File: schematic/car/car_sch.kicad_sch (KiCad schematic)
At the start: 12 parts, among them J1 Led, J10 Motor-PWR-IN, J2 Servo, J3 NRF-Power, J4 Accel, J5 Micro-Power-IN, J6 MOTOR-CTRL, J7 MOTOR-PWR-OUT, J8 Horn, J9 Powers, U1 ARDUINO_PRO_MINI, U2 NRF24L01_Breakout

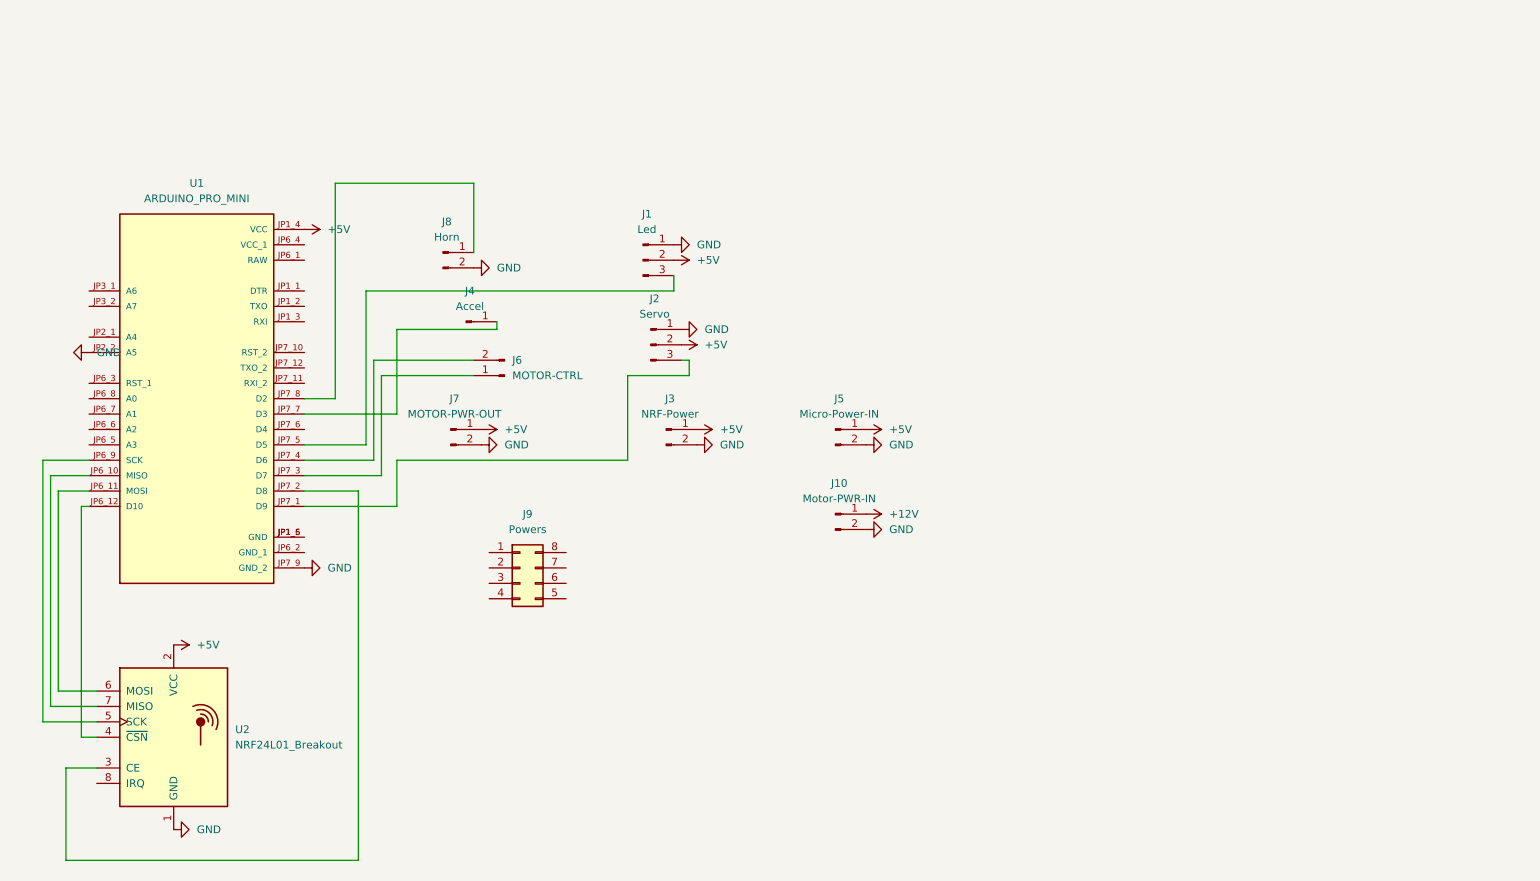
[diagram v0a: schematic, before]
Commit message: drv8833
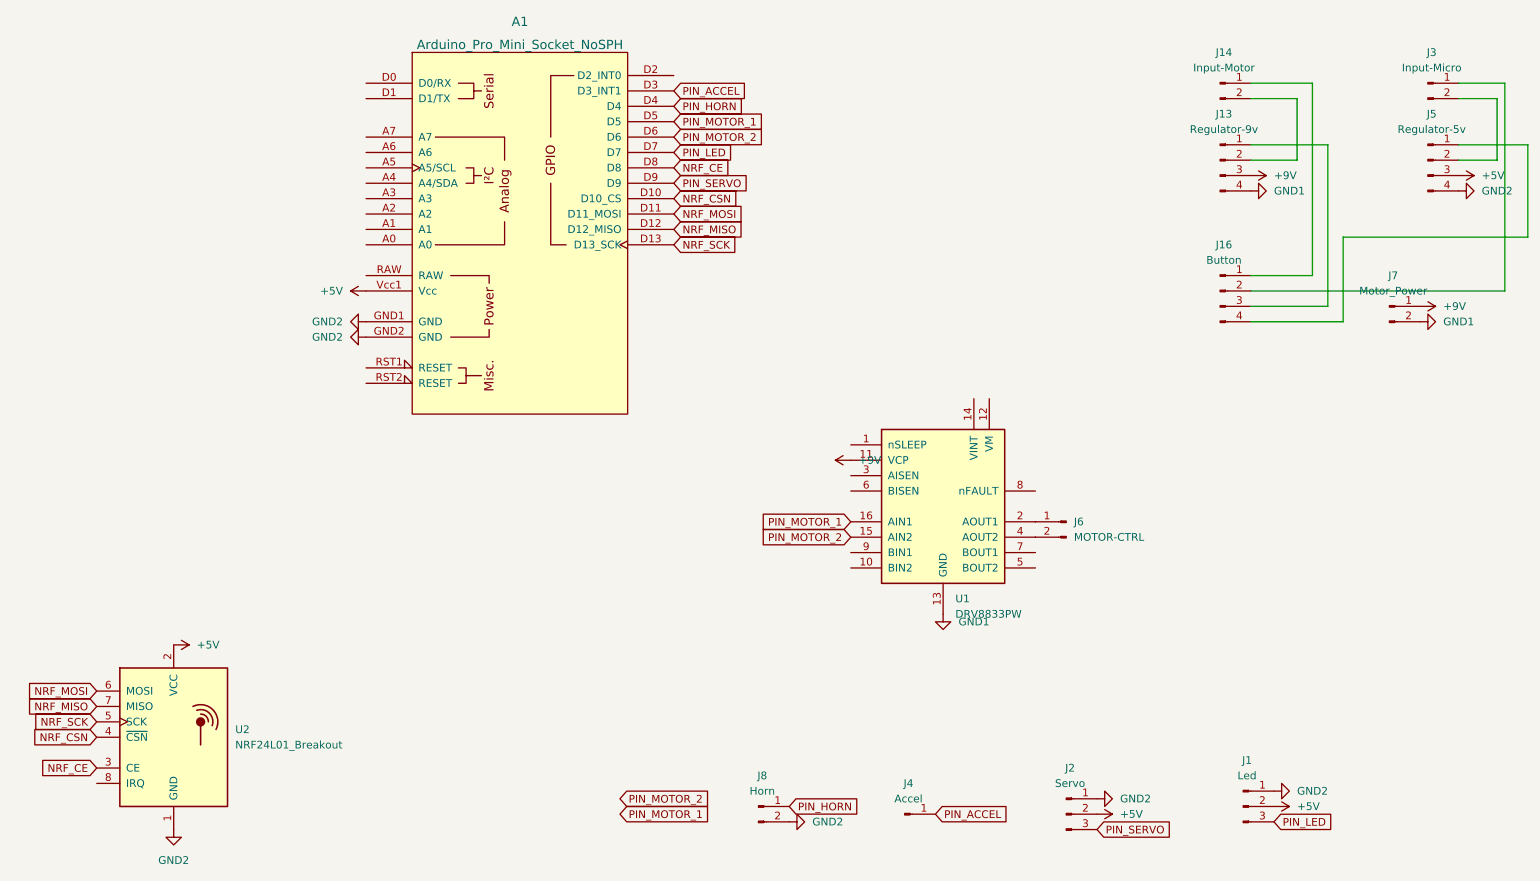
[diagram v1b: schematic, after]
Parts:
- removed J10: Motor-PWR-IN, Connector_PinHeader_2.54mm:PinHeader_1x02_P2.54mm_Vertical, symbol Connector:Conn_01x02_Male
- removed J5: Micro-Power-IN, Connector_PinHeader_2.54mm:PinHeader_1x02_P2.54mm_Vertical, symbol Connector:Conn_01x02_Male
- removed J9: Powers, Connector_PinHeader_2.54mm:PinHeader_2x04_P2.54mm_Vertical, symbol Connector_Generic:Conn_02x04_Counter_Clockwise
- removed U1: ARDUINO_PRO_MINI, MODULE_ARDUINO_PRO_MINI, symbol Arduino pro mini:ARDUINO_PRO_MINI
- added A1: Arduino_Pro_Mini_Socket_NoSPH, PCM_arduino-library:Arduino_Pro_Mini_Socket_NoSPH, symbol PCM_arduino-library:Arduino_Pro_Mini_Socket_NoSPH
- added J13: Regulator-9v, Connector_PinHeader_2.54mm:PinHeader_2x02_P2.54mm_Vertical, symbol Connector:Conn_01x04_Male
- added J14: Input-Motor, Connector_PinHeader_2.54mm:PinHeader_1x02_P2.54mm_Vertical, symbol Connector:Conn_01x02_Male
- added J16: Button, Connector_PinHeader_2.54mm:PinHeader_2x02_P2.54mm_Vertical, symbol Connector:Conn_01x04_Male
- added J5: Regulator-5v, Connector_PinHeader_2.54mm:PinHeader_2x02_P2.54mm_Vertical, symbol Connector:Conn_01x04_Male
- added U1: DRV8833PW, Package_SO:TSSOP-16_4.4x5mm_P0.65mm, symbol Driver_Motor:DRV8833PW
- J3: value NRF-Power -> Input-Micro
- J7: value MOTOR-PWR-OUT -> Motor_Power
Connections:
- net +5V: now also A1.Vcc1 (Vcc), J5.3 (Pin_3); no longer J3.1 (Pin_1), J7.1 (Pin_1)
- net NRF_MISO: now reaches U2.7 (MISO)
- net NRF_MISO: now also A1.D12 (D12_MISO)
- net NRF_MOSI: now reaches U2.6 (MOSI)
- net NRF_MOSI: now also A1.D11 (D11_MOSI)
- net NRF_CSN: now reaches U2.4 (~{CSN})
- net NRF_CSN: now also A1.D10 (D10_CS)
- net NRF_SCK: now reaches U2.5 (SCK)
- net NRF_SCK: now also A1.D13 (D13_SCK)
- net PIN_SERVO: now reaches J2.3 (Pin_3)
- net PIN_SERVO: now also A1.D9
- net NRF_CE: now reaches U2.3 (CE)
- net NRF_CE: now also A1.D8
- net at J6.1 (Pin_1): now also U1.2 (AOUT1)
- net at J6.2 (Pin_2): now also U1.4 (AOUT2)
- net PIN_LED: now reaches J1.3 (Pin_3)
- net PIN_LED: now also A1.D7
- net PIN_ACCEL: now reaches J4.1 (Pin_1)
- net PIN_ACCEL: now also A1.D3 (D3_INT1)
- net PIN_HORN: now reaches J8.1 (Pin_1)
- net PIN_HORN: now also A1.D4
- net GND renamed GND2
- net GND2: now also A1.GND1 (GND), A1.GND2 (GND), J5.4 (Pin_4); no longer J3.2 (Pin_2), J7.2 (Pin_2)
- new net: J16.2 (Pin_2), J3.1 (Pin_1)
- new net: J3.2 (Pin_2), J5.2 (Pin_2)
- new net: J13.1 (Pin_1), J16.3 (Pin_3)
- new net: J13.2 (Pin_2), J14.2 (Pin_2)
- new net: J14.1 (Pin_1), J16.1 (Pin_1)
- new net: J16.4 (Pin_4), J5.1 (Pin_1)
- new net +9V: J13.3 (Pin_3), J7.1 (Pin_1), U1.11 (VCP)
- new net GND1: J13.4 (Pin_4), J7.2 (Pin_2), U1.13 (GND)
- new net PIN_MOTOR_1: A1.D5, U1.16 (AIN1)
- new net PIN_MOTOR_2: A1.D6, U1.15 (AIN2)
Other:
- moved on the sheet: J1, J2, J4, J6, J8
